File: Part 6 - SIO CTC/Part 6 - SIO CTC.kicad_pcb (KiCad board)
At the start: 2 copper layers, 100 x 100 mm, 33 parts, among them J1 EDGE, J2 EXT LCD, J3 USB B, J4 DB9-F, U1 74HC563, U2 Z84C3010, U3 74AHC138, U4 Z84C4010, U5 Z84C4010, U6 MCP2221A, U7 MAX232

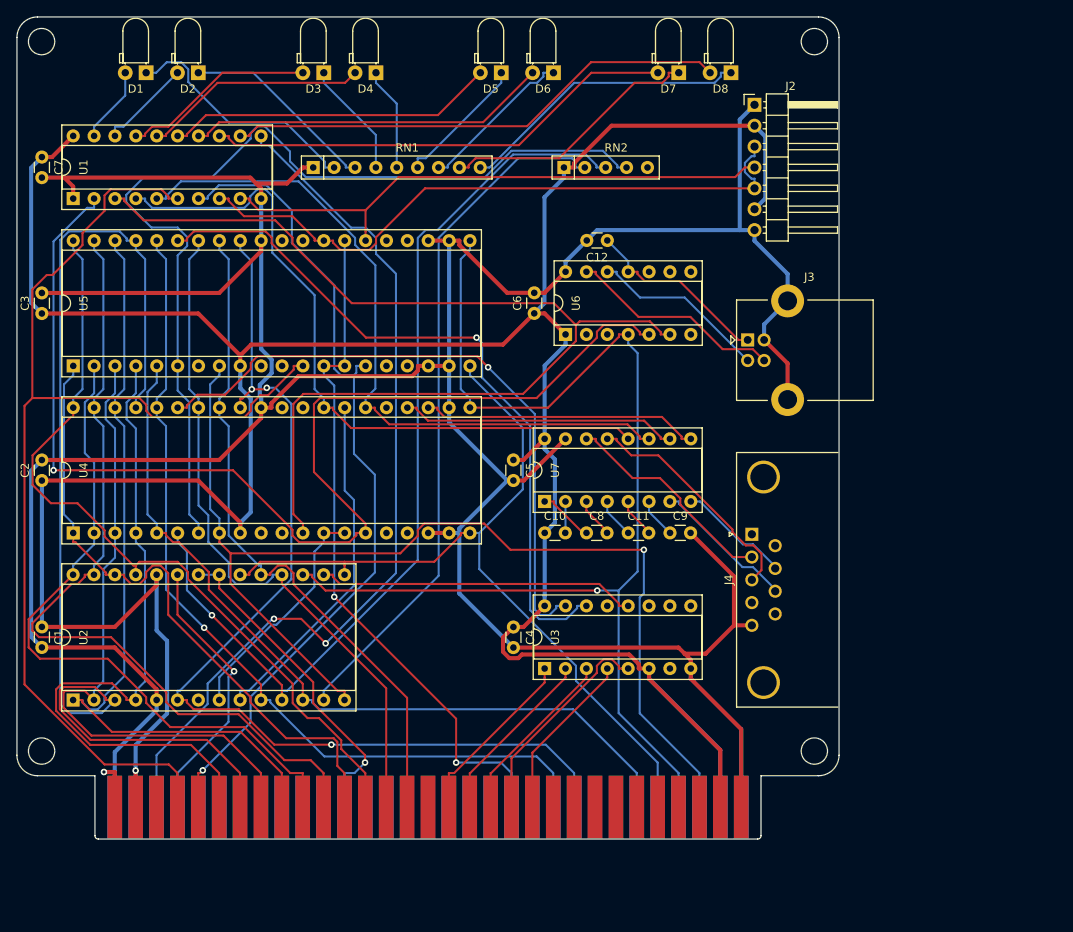
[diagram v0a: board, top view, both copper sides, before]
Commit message: Long time backup
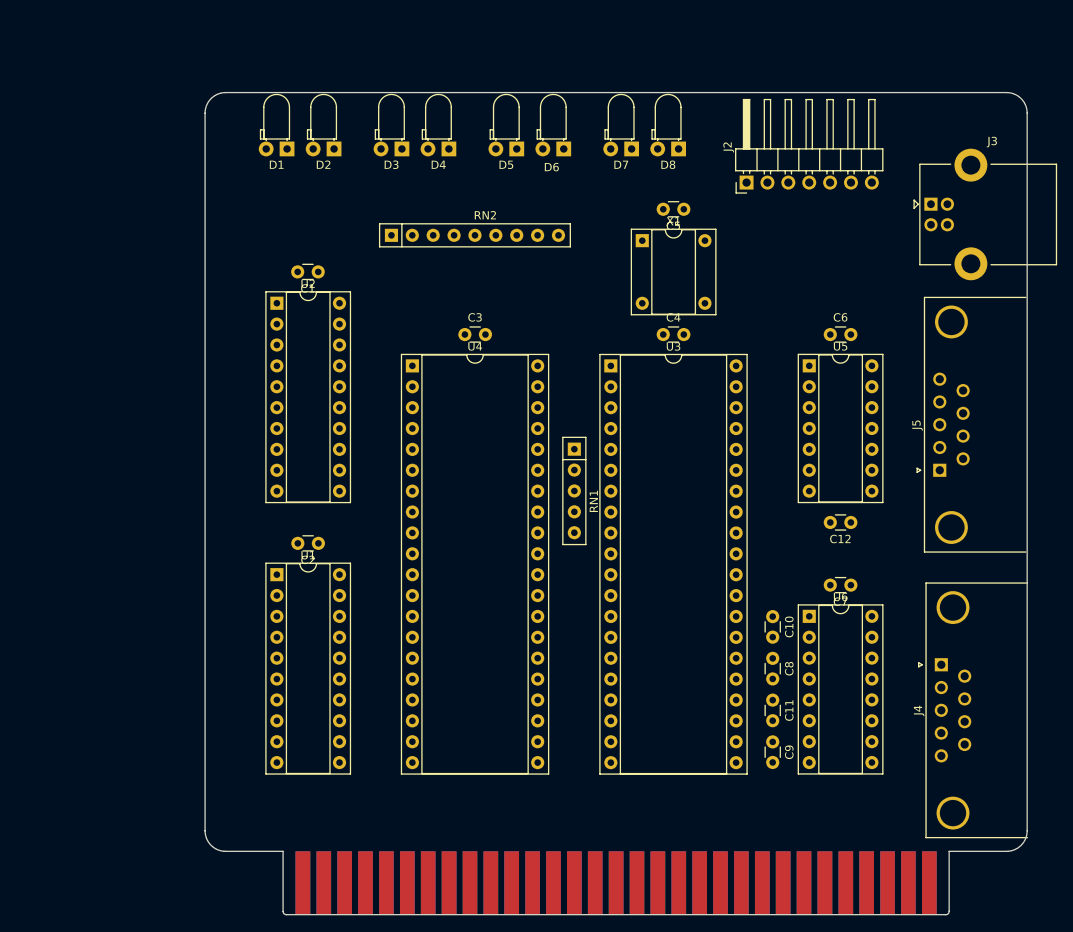
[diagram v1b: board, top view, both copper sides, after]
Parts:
- removed U7: MAX232, Package_DIP:DIP-16_W7.62mm_Socket
- added J5: DB9-M, Connector_Dsub:DSUB-9_Male_Horizontal_P2.77x2.84mm_EdgePinOffset7.70mm_Housed_MountingHolesOffset9.12mm, F.Cu at (181.6, 99.1)
- added X1: 1.8432MHz, 0 - Library:DIP-8-4_W7.62mm_Oscillator_Socket, F.Cu at (145.4, 71.1)
- J1: footprint 0_Z80_Library:BUS_XT -> 0 - Library:BUS_XT
- RN1: value 220 -> 3K3; footprint Resistor_THT:R_Array_SIP9 -> Resistor_THT:R_Array_SIP5
- RN2: value 3K3 -> 330; footprint Resistor_THT:R_Array_SIP5 -> Resistor_THT:R_Array_SIP9
- U1: value 74HC563 -> ATF16V8B
- U2: value Z84C3010 -> 74HC563; footprint Package_DIP:DIP-28_W15.24mm_Socket -> Package_DIP:DIP-20_W7.62mm_Socket
- U3: value 74AHC138 -> Z84C4010; footprint Package_DIP:DIP-16_W7.62mm_Socket -> Package_DIP:DIP-40_W15.24mm_Socket
- U5: value Z84C4010 -> MCP2221A; footprint Package_DIP:DIP-40_W15.24mm_Socket -> Package_DIP:DIP-14_W7.62mm_Socket
- U6: value MCP2221A -> MAX232; footprint Package_DIP:DIP-14_W7.62mm_Socket -> Package_DIP:DIP-16_W7.62mm_Socket
- moved C7 111.3 mm to (170.8, 113.0), turned to 180 degrees
- moved U5 89.5 mm to (165.7, 86.4), turned to 0 degrees
- moved C1 54.7 mm to (106.0, 74.9), turned to 180 degrees
- moved U2 54.3 mm to (101.0, 78.7), turned to 0 degrees
- moved U1 52.0 mm to (101.0, 111.8), turned to 0 degrees
- moved C3 51.5 mm to (123.8, 82.5), turned to 0 degrees
- moved RN1 46.7 mm to (137.2, 96.5), turned to -90 degrees
- moved U4 46.0 mm to (117.5, 86.4), turned to 0 degrees
- moved U6 45.3 mm to (165.7, 116.8), turned to 0 degrees
- moved C12 45.3 mm to (170.8, 105.4)
- moved C4 40.0 mm to (148.0, 82.5), turned to 0 degrees
- moved U3 37.7 mm to (141.6, 86.4), turned to 0 degrees
- moved C5 36.9 mm to (150.5, 67.3), turned to 180 degrees
- moved C6 36.1 mm to (168.3, 82.5), turned to 0 degrees
- moved C2 34.5 mm to (106.0, 108.0), turned to 180 degrees
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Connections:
- J1 pad 10: /A8 -> unconnected-(J1-Pad10)
- J1 pad 29: /+3V3 -> unconnected-(J1-Pad29)
- J1 pad 3: /A15 -> unconnected-(J1-Pad3)
- J1 pad 38: /~{MREQ} -> unconnected-(J1-Pad38)
- J1 pad 39: /~{WR} -> unconnected-(J1-Pad39)
- J1 pad 4: /A14 -> unconnected-(J1-Pad4)
- J1 pad 42: /~{MR} -> unconnected-(J1-Pad42)
- J1 pad 43: /CLK2 -> unconnected-(J1-Pad43)
- J1 pad 44: /~{BUSAK} -> unconnected-(J1-Pad44)
- J1 pad 45: /~{HALT} -> unconnected-(J1-Pad45)
- J1 pad 46: /~{BUSRQ} -> unconnected-(J1-Pad46)
- J1 pad 47: /~{WAIT} -> unconnected-(J1-Pad47)
- J1 pad 48: /~{NMI} -> unconnected-(J1-Pad48)
- J1 pad 49: /~{CLK_DIS} -> unconnected-(J1-Pad49)
- J1 pad 5: /A13 -> unconnected-(J1-Pad5)
- J1 pad 50: /~{CLK_SEL} -> unconnected-(J1-Pad50)
- J1 pad 51: /CLK4 -> unconnected-(J1-Pad51)
- J1 pad 52: /~{PWR_UP} -> unconnected-(J1-Pad52)
- J1 pad 53: /USER1 -> unconnected-(J1-Pad53)
- J1 pad 54: /USER2 -> unconnected-(J1-Pad54)
- J1 pad 55: /USER3 -> unconnected-(J1-Pad55)
- J1 pad 56: /USER4 -> unconnected-(J1-Pad56)
- J1 pad 57: /~{IORD} -> unconnected-(J1-Pad57)
- J1 pad 58: /~{IOWR} -> unconnected-(J1-Pad58)
- J1 pad 59: /CLK1 -> unconnected-(J1-Pad59)
- J1 pad 6: /A12 -> unconnected-(J1-Pad6)
- J1 pad 60: /~{CLK} -> unconnected-(J1-Pad60)
- J1 pad 7: /A11 -> unconnected-(J1-Pad7)
- J1 pad 8: /A10 -> unconnected-(J1-Pad8)
- J1 pad 9: /A9 -> unconnected-(J1-Pad9)
- J3 pad 1: Net-(C12-Pad1) -> unconnected-(J3-Pad1)
- RN1 pad 1: GND -> +5V
- RN1 pad 2: Net-(D1-Pad1) -> /SIO_IEI
- RN1 pad 3: Net-(D2-Pad1) -> /SIO_IEO
- RN1 pad 4: Net-(D3-Pad1) -> /SDA
- RN1 pad 5: Net-(D4-Pad1) -> /SCL
- RN2 pad 1: +5V -> GND
- RN2 pad 2: /CTC_IEI -> Net-(D1-Pad1)
- RN2 pad 3: /CTC_IEO -> Net-(D2-Pad1)
- RN2 pad 4: /SIO_IEO -> Net-(D3-Pad1)
- RN2 pad 5: unconnected-(RN2-Pad5) -> Net-(D4-Pad1)
- U1 pad 1: GND -> /~{IORQ}
- U1 pad 11: /~{CLK} -> GND
- U1 pad 12: Net-(D8-Pad2) -> unconnected-(U1-Pad12)
- U1 pad 13: Net-(D7-Pad2) -> unconnected-(U1-Pad13)
- U1 pad 14: Net-(D6-Pad2) -> unconnected-(U1-Pad14)
- U1 pad 15: Net-(D5-Pad2) -> unconnected-(U1-Pad15)
- U1 pad 16: Net-(D4-Pad2) -> unconnected-(U1-Pad16)
- U1 pad 17: Net-(D3-Pad2) -> unconnected-(U1-Pad17)
- U1 pad 18: Net-(D2-Pad2) -> /~{SIO2CS}
- U1 pad 19: Net-(D1-Pad2) -> /~{SIO1CS}
- U1 pad 2: /RxA -> /~{M1}
- U1 pad 3: /TxA -> /A2
- U1 pad 4: /RxB -> /A3
- U1 pad 5: /TxB -> /A4
- U1 pad 6: /RX -> /A5
- U1 pad 7: /TX -> /A6
- U1 pad 8: /LCD_Rx -> /A7
- U1 pad 9: /LCD_Tx -> GND
- U2 pad 1: /D4 -> GND
- U2 pad 10: /~{IORQ} -> GND
- U2 pad 11: /CTC_IEO -> +5V
- U2 pad 12: /~{INT} -> Net-(D8-Pad2)
- U2 pad 13: /CTC_IEI -> Net-(D7-Pad2)
- U2 pad 14: /~{M1} -> Net-(D6-Pad2)
- U2 pad 15: /CLK -> Net-(D5-Pad2)
- U2 pad 16: /~{CTC_CS} -> Net-(D4-Pad2)
- U2 pad 17: /~{RESET} -> Net-(D3-Pad2)
- U2 pad 18: /A0 -> Net-(D2-Pad2)
- U2 pad 19: /A1 -> Net-(D1-Pad2)
- U2 pad 2: /D5 -> /RxA
- U2 pad 20: /CLK -> +5V
- U2 pad 3: /D6 -> /TxA
- U2 pad 4: /D7 -> /RxB
- U2 pad 5: GND -> /TxB
- U2 pad 6: /~{RD} -> /RX
- U2 pad 7: unconnected-(U2-Pad7) -> /TX
- U2 pad 8: /CTCCLKA -> /LCD_Rx
- U2 pad 9: /CTCCLKB -> /LCD_Tx
- U3 pad 1: /A3 -> /D1
- U3 pad 12: /~{CTC_CS} -> /TxA
- U3 pad 13: unconnected-(U3-Pad13) -> /CLKSIO
- U3 pad 14: /~{SIO2_CS} -> /CLKSIO
- U3 pad 15: /~{SIO1_CS} -> /RxA
- U3 pad 16: +5V -> unconnected-(U3-Pad16)
- U3 pad 2: /A4 -> /D3
- U3 pad 3: /A5 -> /D5
- U3 pad 4: /A7 -> /D7
- U3 pad 5: /A6 -> /~{INT}
- U3 pad 6: +5V -> /SIO_IEI
- U3 pad 7: unconnected-(U3-Pad7) -> /SIO_IEO
- U3 pad 8: GND -> /~{M1}
- U3 pad 9: unconnected-(U3-Pad9) -> +5V
- U4 pad 12: /TxA -> /RX
- U4 pad 13: /CTCCLKA -> /CLKSIO
- U4 pad 14: /CTCCLKA -> /CLKSIO
- U4 pad 15: /RxA -> /TX
- U4 pad 23: Net-(U4-Pad23) -> GND
- U4 pad 24: Net-(U4-Pad24) -> unconnected-(U4-Pad24)
- U4 pad 26: /TxB -> /LCD_Tx
- U4 pad 27: /CTCCLKB -> /CLKSIO
- U4 pad 28: /RxB -> /LCD_Rx
- U4 pad 35: /~{SIO1_CS} -> /~{SIO2CS}
- U4 pad 6: /CTC_IEO -> /SIO_IEO
- U4 pad 7: /SIO_IEO -> unconnected-(U4-Pad7)
- U5 pad 1: /D1 -> +5V
- U5 pad 10: unconnected-(U5-Pad10) -> /SCL
- U5 pad 11: unconnected-(U5-Pad11) -> Net-(C12-Pad1)
- U5 pad 12: /RX -> Net-(J3-Pad2)
- U5 pad 13: /CLK2 -> Net-(J3-Pad3)
- U5 pad 14: /CLK2 -> GND
- U5 pad 2: /D3 -> unconnected-(U5-Pad2)
- U5 pad 3: /D5 -> unconnected-(U5-Pad3)
- U5 pad 4: /D7 -> /~{RESET}
- U5 pad 5: /~{INT} -> /RxA
- U5 pad 6: /SIO_IEO -> /TxA
- U5 pad 8: /~{M1} -> unconnected-(U5-Pad8)
- U5 pad 9: +5V -> /SDA
- U6 pad 1: +5V -> Net-(C8-Pad1)
- U6 pad 10: unconnected-(U6-Pad10) -> Net-(U3-Pad24)
- U6 pad 11: Net-(C12-Pad1) -> /TxB
- U6 pad 12: Net-(J3-Pad2) -> /RxB
- U6 pad 13: Net-(J3-Pad3) -> Net-(J4-Pad3)
- U6 pad 14: GND -> Net-(J4-Pad2)
- U6 pad 2: /RxDATA -> Net-(C10-Pad2)
- U6 pad 3: /TxDATA -> Net-(C8-Pad2)
- U6 pad 4: /~{RESET} -> Net-(C11-Pad1)
- U6 pad 5: /RxA -> Net-(C11-Pad2)
- U6 pad 6: /TxA -> Net-(C9-Pad1)
- U6 pad 7: unconnected-(U6-Pad7) -> Net-(J4-Pad8)
- U6 pad 8: unconnected-(U6-Pad8) -> Net-(J4-Pad7)
- U6 pad 9: unconnected-(U6-Pad9) -> Net-(U3-Pad23)
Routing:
- net GND: track 457.6 -> 0.00 mm, vias 1 -> 0
- net +5V: track 378.7 -> 0.00 mm, vias 1 -> 0
- net /~{RESET}: track 145.7 -> 0.00 mm, vias 1 -> 0
- net /RxA: track 142.3 -> 0.00 mm, vias 1 -> 0
- net /RX: track 138.5 -> 0.00 mm
- net /~{M1}: track 136.4 -> 0.00 mm, vias 1 -> 0
- net /D6: track 135.0 -> 0.00 mm
- net /TxA: track 131.2 -> 0.00 mm
- net /~{RD}: track 125.5 -> 0.00 mm, vias 3 -> 0
- net /SIO_IEO: track 117.9 -> 0.00 mm
- net /CTC_IEO: track 116.9 -> 0.00 mm, vias 1 -> 0
- net /~{CLK}: track 110.1 -> 0.00 mm, vias 2 -> 0
- net /~{IORQ}: track 105.6 -> 0.00 mm, vias 1 -> 0
- net /TX: track 102.6 -> 0.00 mm, vias 1 -> 0
- net /D2: track 101.0 -> 0.00 mm
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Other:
- outline, holes or cut-outs redrawn
